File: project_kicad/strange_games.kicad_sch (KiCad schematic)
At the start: 93 parts, among them J1 Display, M1 Motor_DC, Q1 Si2302A, Q3 Si2302A, Q4 Q_Photo, SW1 SW_Push, SW10 SW_Push, SW11 SW_Push, SW2 SW_Push, SW3 SW_Push, SW4 SW_Push, SW5 SW_Push, SW6 SW_Push, SW7 SW_Push, SW8 SW_Push, SW9 SW_Push, U1 charge controller, U2 boost converter, U3 LDL1117S33R, U4 ESP32-DEVKIT-V1, U5 TMP112xxDRL, U6 vibrating_sensor, U7 LSM6DS3, U8 MQ-135 gas sensor

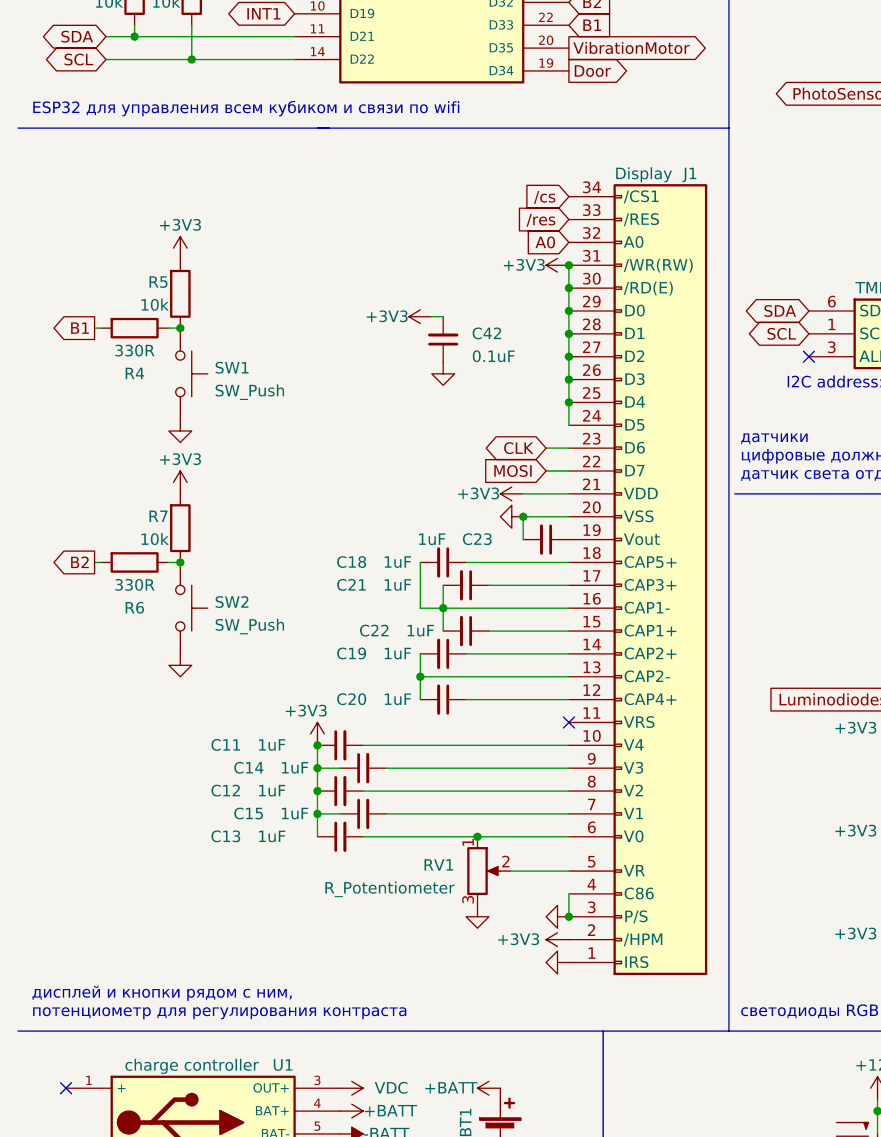
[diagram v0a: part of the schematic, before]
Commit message: I need to remaster everything
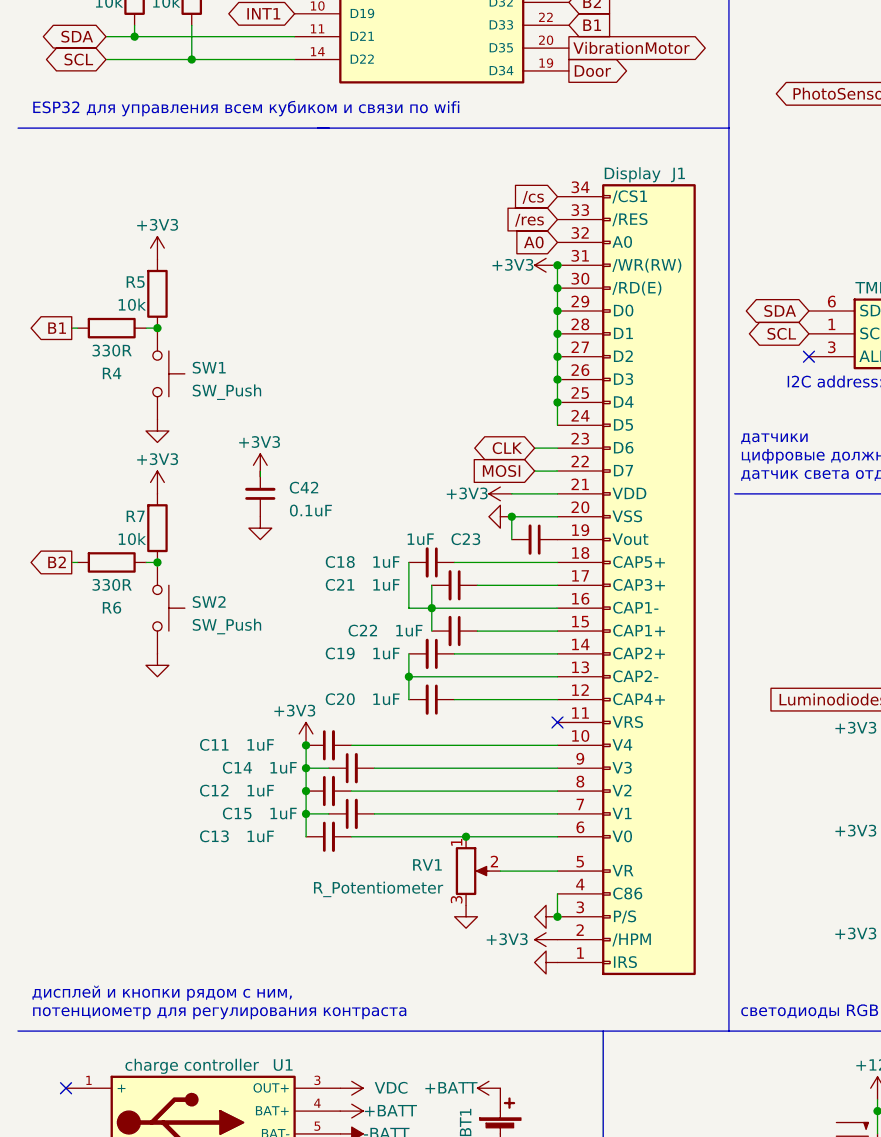
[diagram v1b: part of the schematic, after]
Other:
- moved on the sheet: C11, C12, C13, C14, C15, C18, C19, C20, C21, C22, C23, C42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
